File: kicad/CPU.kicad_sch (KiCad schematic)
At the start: 22 parts, among them J1 Free pin, J2 Free pins, J3 Free pin, J4 Free pin, J5 Free pin, U10 GAL22V10, U11 AS6C4008-55PCN, U12 AS6C4008-55PCN, U12 GAL22V10, U5 SST39SF040, U6 SST39SF040, U7 68010P10

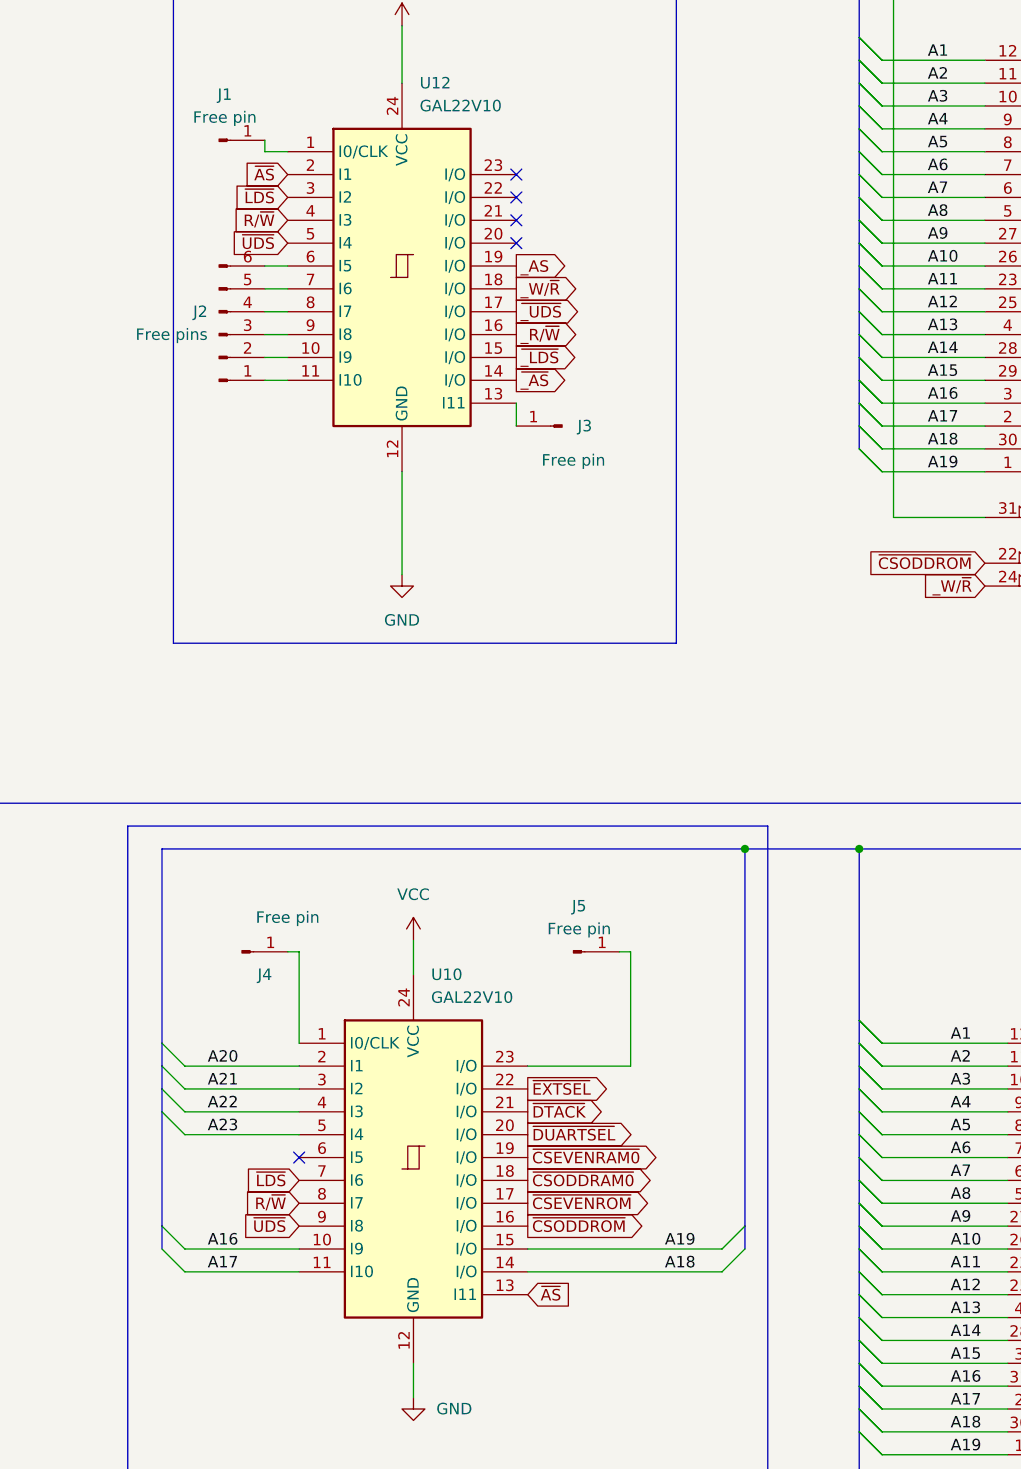
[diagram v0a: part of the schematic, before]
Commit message: fiddlign with placement
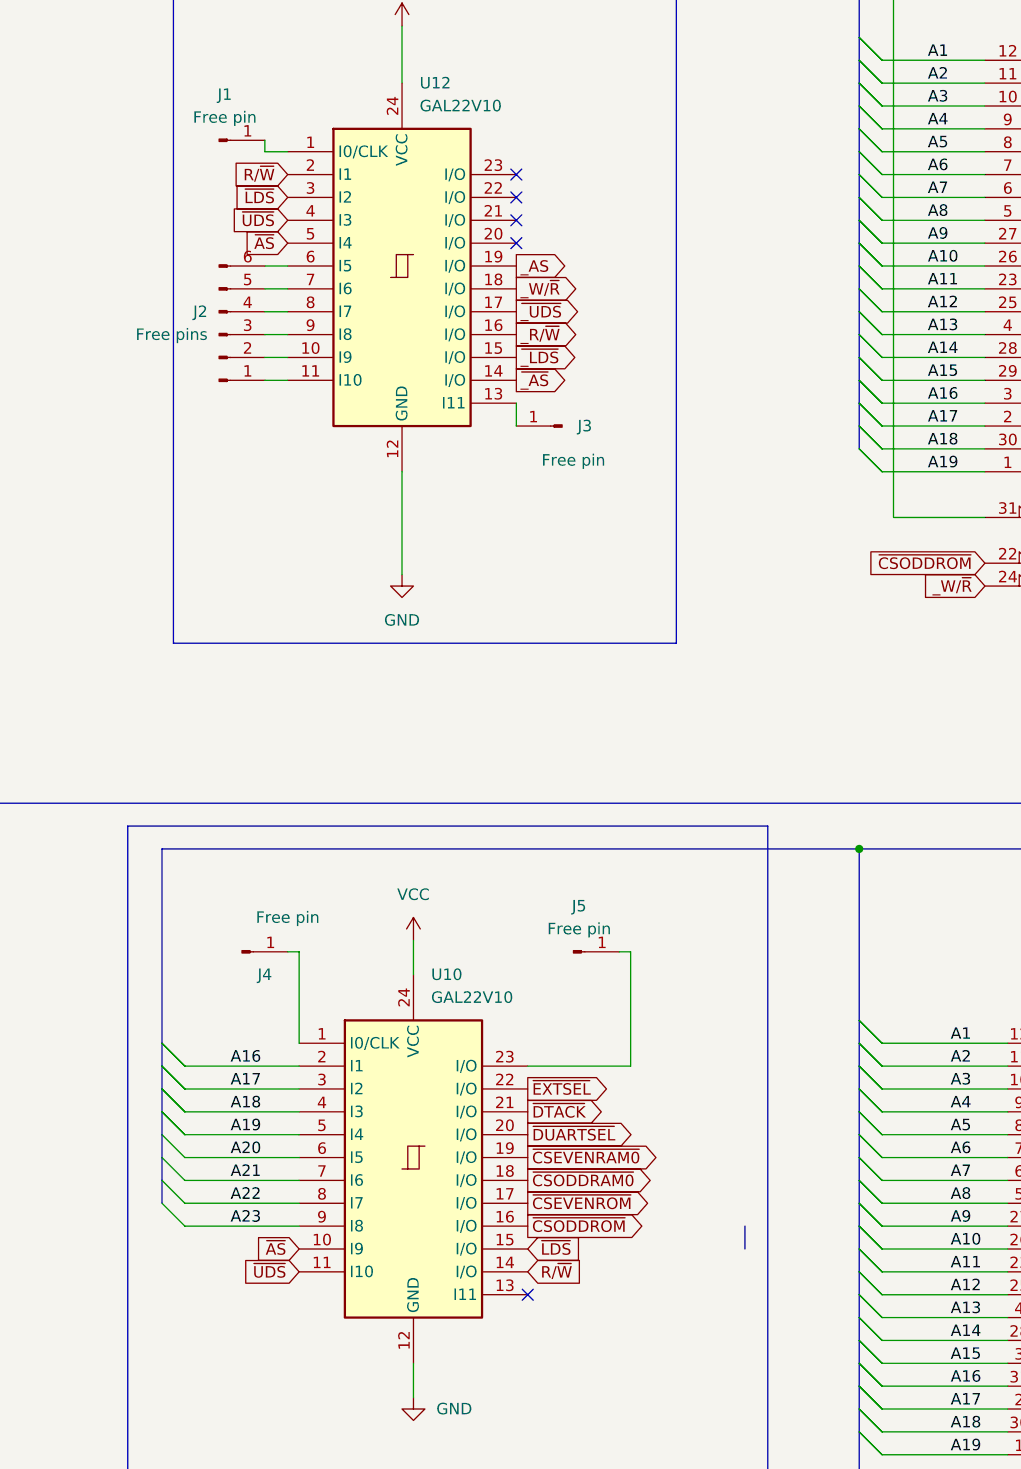
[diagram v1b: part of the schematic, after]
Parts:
- C6, C7: footprint Capacitor_THT:CP_Radial_D5.0mm_P2.50mm -> Capacitor_THT:C_Disc_D5.0mm_W2.5mm_P2.50mm
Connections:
- net A16: now also U10.2 (I1); no longer U10.10 (I9)
- net A17: now also U10.3 (I2); no longer U10.11 (I10)
- net A18: now also U10.4 (I3); no longer U10.14 (I/O)
- net A19: now also U10.5 (I4); no longer U10.15 (I/O)
- net A20: now also U10.6 (I5); no longer U10.2 (I1)
- net A21: now also U10.7 (I6); no longer U10.3 (I2)
- net A22: now also U10.8 (I7); no longer U10.4 (I3)
- net A23: now also U10.9 (I8); no longer U10.5 (I4)
- net R/~{W}: now also U10.14 (I/O), U12.2 (I1); no longer U10.8 (I7), U12.4 (I3)
- net ~{AS}: now also U10.10 (I9), U12.5 (I4); no longer U10.13 (I11), U12.2 (I1)
- net ~{LDS}: now also U10.15 (I/O); no longer U10.7 (I6)
- net ~{UDS}: now also U10.11 (I10), U12.4 (I3); no longer U10.9 (I8), U12.5 (I4)

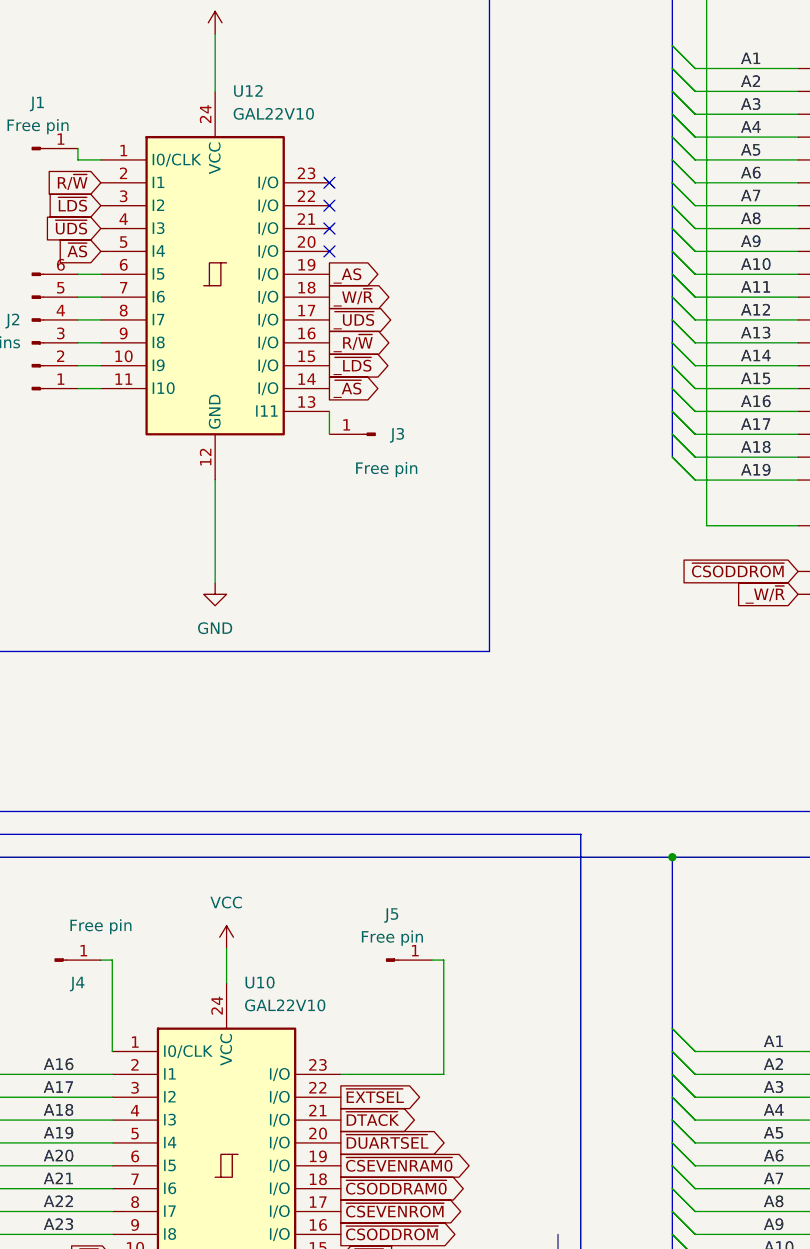
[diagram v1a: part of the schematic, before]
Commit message: got irq to work
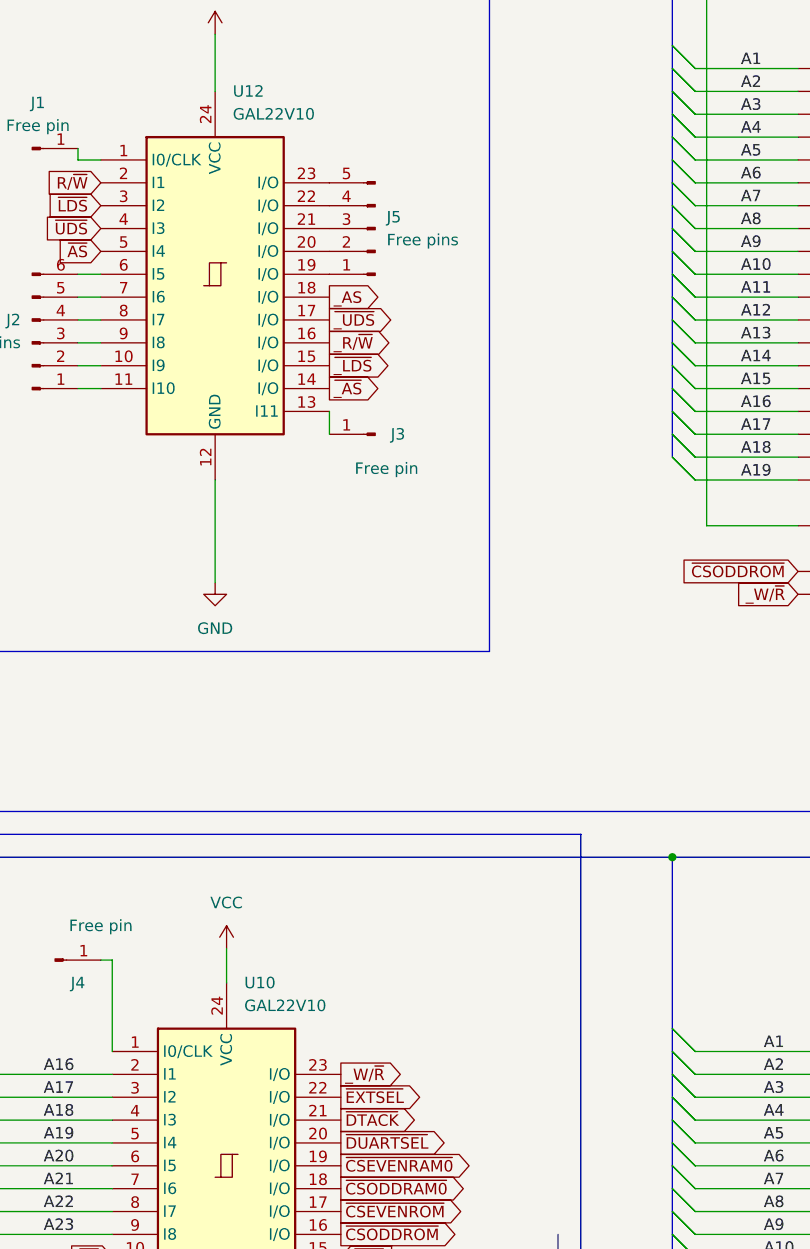
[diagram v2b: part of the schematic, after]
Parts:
- removed J5: Free pin, Connector_PinSocket_2.54mm:PinSocket_1x01_P2.54mm_Vertical, symbol Connector:Conn_01x01_Pin
- added J5: Free pins, Connector_PinSocket_2.54mm:PinSocket_1x05_P2.54mm_Vertical, symbol Connector:Conn_01x05_Pin
- U5, U6: footprint Package_DIP:DIP-32_W15.24mm_Socket -> Socket:DIP_Socket-32_W11.9_W12.7_W15.24_W17.78_W18.5_3M_232-1285-00-0602J
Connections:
- net _AS: now also U12.18 (I/O); no longer U12.19 (I/O)
- net _W/~{R}: now also U10.23 (I/O); no longer U12.18 (I/O)
- net at U12.20 (I/O): now also J5.2 (Pin_2)
- net at U12.21 (I/O): now also J5.3 (Pin_3)
- net at U12.22 (I/O): now also J5.4 (Pin_4)
- net at U12.23 (I/O): now also J5.5 (Pin_5)
- new net: J5.1 (Pin_1), U12.19 (I/O)
- no-connect marks 7 -> 3
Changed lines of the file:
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@@
   (junction (at 331.47 229.87) (diameter 0) (color 0 0 0 0)
   )
-  (no_connect (at 237.49 64.77))
-  (no_connect (at 237.49 67.31))
   (no_connect (at 40.64 74.93))
   (no_connect (at 238.76 189.23))
-  (no_connect (at 237.49 72.39))
-  (no_connect (at 237.49 69.85))
   (no_connect (at 40.64 52.07))
   (bus_entry (at 275.59 57.15) (size 2.54 2.54)
@@
     (stroke (width 0) (type default))
   )
-  (wire (pts (xy 250.19 151.13) (xy 250.19 163.83))
-    (stroke (width 0) (type default))
-  )
   (bus (pts (xy 101.6 102.87) (xy 101.6 105.41))
     (stroke (width 0) (type default))
@@
     (stroke (width 0) (type default))
   )
-  (wire (pts (xy 238.76 163.83) (xy 250.19 163.83))
-    (stroke (width 0) (type default))
-  )
   (wire (pts (xy 39.37 102.87) (xy 40.64 102.87))
     (stroke (width 0) (type default))
@@
     (stroke (width 0) (type default))
   )
-  (wire (pts (xy 248.92 151.13) (xy 250.19 151.13))
-    (stroke (width 0) (type default))
-  )
   (bus (pts (xy 275.59 87.63) (xy 275.59 90.17))
     (stroke (width 0) (type default))
@@
     (effects (font (size 1.27 1.27)) (justify left bottom))
   )
-  (label "A16" (at 205.74 163.83 0)
+  (label "A16" (at 205.74 163.83 0) (fields_autoplaced)
     (effects (font (size 1.27 1.27)) (justify left bottom))
   )
@@
     (effects (font (size 1.27 1.27)) (justify left bottom))
   )
-  (label "A20" (at 205.74 173.99 0)
+  (label "A20" (at 205.74 173.99 0) (fields_autoplaced)
     (effects (font (size 1.27 1.27)) (justify left bottom))
   )
@@
     (effects (font (size 1.27 1.27)) (justify left bottom))
   )
-  (label "A18" (at 205.74 168.91 0)
+  (label "A18" (at 205.74 168.91 0) (fields_autoplaced)
     (effects (font (size 1.27 1.27)) (justify left bottom))
   )
@@
     (effects (font (size 1.27 1.27)) (justify left bottom))
   )
-  (label "A22" (at 205.74 179.07 0)
+  (label "A22" (at 205.74 179.07 0) (fields_autoplaced)
     (effects (font (size 1.27 1.27)) (justify left bottom))
   )
@@
     (effects (font (size 1.27 1.27)) (justify left bottom))
   )
-  (label "A21" (at 205.74 176.53 0)
+  (label "A21" (at 205.74 176.53 0) (fields_autoplaced)
     (effects (font (size 1.27 1.27)) (justify left bottom))
   )
@@
     (effects (font (size 1.27 1.27)) (justify left bottom))
   )
-  (label "A19" (at 205.74 171.45 0)
+  (label "A19" (at 205.74 171.45 0) (fields_autoplaced)
     (effects (font (size 1.27 1.27)) (justify left bottom))
   )
@@
     (effects (font (size 1.27 1.27)) (justify left bottom))
   )
-  (label "A23" (at 205.74 181.61 0)
+  (label "A23" (at 205.74 181.61 0) (fields_autoplaced)
     (effects (font (size 1.27 1.27)) (justify left bottom))
   )
@@
     (effects (font (size 1.27 1.27)) (justify left bottom))
   )
-  (label "A17" (at 205.74 166.37 0)
+  (label "A17" (at 205.74 166.37 0) (fields_autoplaced)
     (effects (font (size 1.27 1.27)) (justify left bottom))
   )
@@
     )
   )
-  (global_label "_W{slash}~{R}" (shape output) (at 237.49 77.47 0) (fields_autoplaced)
+  (global_label "_W{slash}~{R}" (shape output) (at 238.76 163.83 0) (fields_autoplaced)
     (effects (font (size 1.27 1.27)) (justify left))
-    (property "Intersheetrefs" "${INTERSHEET_REFS}" (at 245.4153 77.47 0)
+    (property "Intersheetrefs" "${INTERSHEET_REFS}" (at 246.6853 163.83 0)
       (effects (font (size 1.27 1.27)) (justify left) hide)
     )
@@
     )
   )
-  (global_label "_AS" (shape output) (at 237.49 74.93 0) (fields_autoplaced)
+  (global_label "_AS" (shape output) (at 237.49 77.47 0) (fields_autoplaced)
     (effects (font (size 1.27 1.27)) (justify left))
-    (property "Intersheetrefs" "${INTERSHEET_REFS}" (at 243.6615 74.93 0)
+    (property "Intersheetrefs" "${INTERSHEET_REFS}" (at 243.6615 77.47 0)
       (effects (font (size 1.27 1.27)) (justify left) hide)
     )
@@
       (effects (font (size 1.27 1.27)))
     )
-    (property "Footprint" "Package_DIP:DIP-32_W15.24mm_Socket" (at 304.8 74.93 0)
+    (property "Footprint" "Socket:DIP_Socket-32_W11.9_W12.7_W15.24_W17.78_W18.5_3M_232-1285-00-0602J" (at 304.8 74.93 0)
       (effects (font (size 1.27 1.27)) hide)
     )
@@
       (effects (font (size 1.27 1.27)))
     )
-    (property "Footprint" "Package_DIP:DIP-32_W15.24mm_Socket" (at 363.22 74.93 0)
+    (property "Footprint" "Socket:DIP_Socket-32_W11.9_W12.7_W15.24_W17.78_W18.5_3M_232-1285-00-0602J" (at 363.22 74.93 0)
       (effects (font (size 1.27 1.27)) hide)
     )
@@
     )
   )
-  (symbol (lib_id "power:VCC") (at 304.8 148.59 0) (unit 1)
+  (symbol (lib_id "Connector:Conn_01x05_Pin") (at 242.57 69.85 180) (unit 1)
     (in_bom yes) (on_board yes) (dnp no) (fields_autoplaced)
-    (property "Reference" "#PWR024" (at 304.8 152.4 0)
-      (effects (font (size 1.27 1.27)) hide)
+    (property "Reference" "J5" (at 243.84 68.58 0)
+      (effects (font (size 1.27 1.27)) (justify right))
     )
-    (property "Value" "VCC" (at 304.8 143.51 0)
-      (effects (font (size 1.27 1.27)))
+    (property "Value" "Free pins" (at 243.84 71.12 0)
+      (effects (font (size 1.27 1.27)) (justify right))
     )
-    (property "Footprint" "" (at 304.8 148.59 0)
+    (property "Footprint" "Connector_PinSocket_2.54mm:PinSocket_1x05_P2.54mm_Vertical" (at 242.57 69.85 0)
       (effects (font (size 1.27 1.27)) hide)
     )
-    (property "Datasheet" "" (at 304.8 148.59 0)
+    (property "Datasheet" "~" (at 242.57 69.85 0)
       (effects (font (size 1.27 1.27)) hide)
     )
     (pin "1")
+    (pin "2")
+    (pin "3")
+    (pin "4")
+    (pin "5")
     (instances
       (project "mb68k"
         (path "/e63e39d7-6ac0-4ffd-8aa3-1841a4541b55/c0b233c3-0354-40a8-9da4-8134543aeba9"
-          (reference "#PWR024") (unit 1)
+          (reference "J5") (unit 1)
         )
       )
     )
   )
-  (symbol (lib_id "power:VCC") (at 363.22 148.59 0) (unit 1)
+  (symbol (lib_id "power:VCC") (at 304.8 148.59 0) (unit 1)
     (in_bom yes) (on_board yes) (dnp no) (fields_autoplaced)
-    (property "Reference" "#PWR025" (at 363.22 152.4 0)
+    (property "Reference" "#PWR024" (at 304.8 152.4 0)
       (effects (font (size 1.27 1.27)) hide)
     )
-    (property "Value" "VCC" (at 363.22 143.51 0)
+    (property "Value" "VCC" (at 304.8 143.51 0)
       (effects (font (size 1.27 1.27)))
     )
-    (property "Footprint" "" (at 363.22 148.59 0)
+    (property "Footprint" "" (at 304.8 148.59 0)
       (effects (font (size 1.27 1.27)) hide)
     )
-    (property "Datasheet" "" (at 363.22 148.59 0)
+    (property "Datasheet" "" (at 304.8 148.59 0)
       (effects (font (size 1.27 1.27)) hide)
     )
@@
       (project "mb68k"
         (path "/e63e39d7-6ac0-4ffd-8aa3-1841a4541b55/c0b233c3-0354-40a8-9da4-8134543aeba9"
-          (reference "#PWR025") (unit 1)
+          (reference "#PWR024") (unit 1)
         )
       )
     )
   )
-  (symbol (lib_id "Connector:Conn_01x01_Pin") (at 243.84 151.13 0) (unit 1)
+  (symbol (lib_id "power:VCC") (at 363.22 148.59 0) (unit 1)
     (in_bom yes) (on_board yes) (dnp no) (fields_autoplaced)
-    (property "Reference" "J5" (at 244.475 146.05 0)
-      (effects (font (size 1.27 1.27)))
+    (property "Reference" "#PWR025" (at 363.22 152.4 0)
+      (effects (font (size 1.27 1.27)) hide)
     )
-    (property "Value" "Free pin" (at 244.475 148.59 0)
+    (property "Value" "VCC" (at 363.22 143.51 0)
       (effects (font (size 1.27 1.27)))
     )
-    (property "Footprint" "Connector_PinSocket_2.54mm:PinSocket_1x01_P2.54mm_Vertical" (at 243.84 151.13 0)
+    (property "Footprint" "" (at 363.22 148.59 0)
       (effects (font (size 1.27 1.27)) hide)
     )
-    (property "Datasheet" "~" (at 243.84 151.13 0)
+    (property "Datasheet" "" (at 363.22 148.59 0)
       (effects (font (size 1.27 1.27)) hide)
     )
@@
       (project "mb68k"
         (path "/e63e39d7-6ac0-4ffd-8aa3-1841a4541b55/c0b233c3-0354-40a8-9da4-8134543aeba9"
-          (reference "J5") (unit 1)
+          (reference "#PWR025") (unit 1)
         )
       )
